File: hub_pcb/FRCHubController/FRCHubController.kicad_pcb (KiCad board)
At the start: 2 copper layers, 60 x 79.5 mm, 20 parts, among them J1 Conn_01x03_Socket, J2 Conn_01x03_Socket, J3 Conn_01x03_Socket, J4 Barrel_Jack_Switch_Pin3Ring, J5 Conn_02x08_Odd_Even, U6 TXB0102DCU

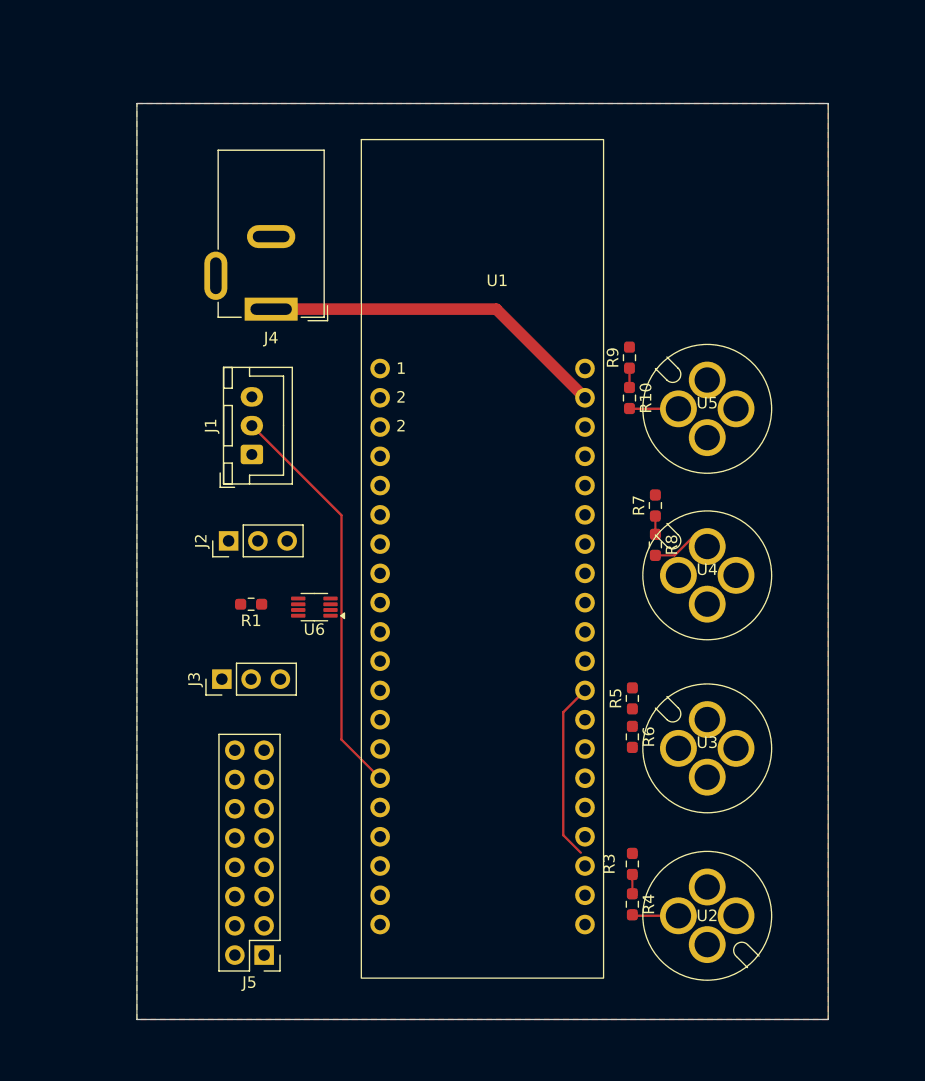
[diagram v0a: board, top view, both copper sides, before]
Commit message: Layout PCB
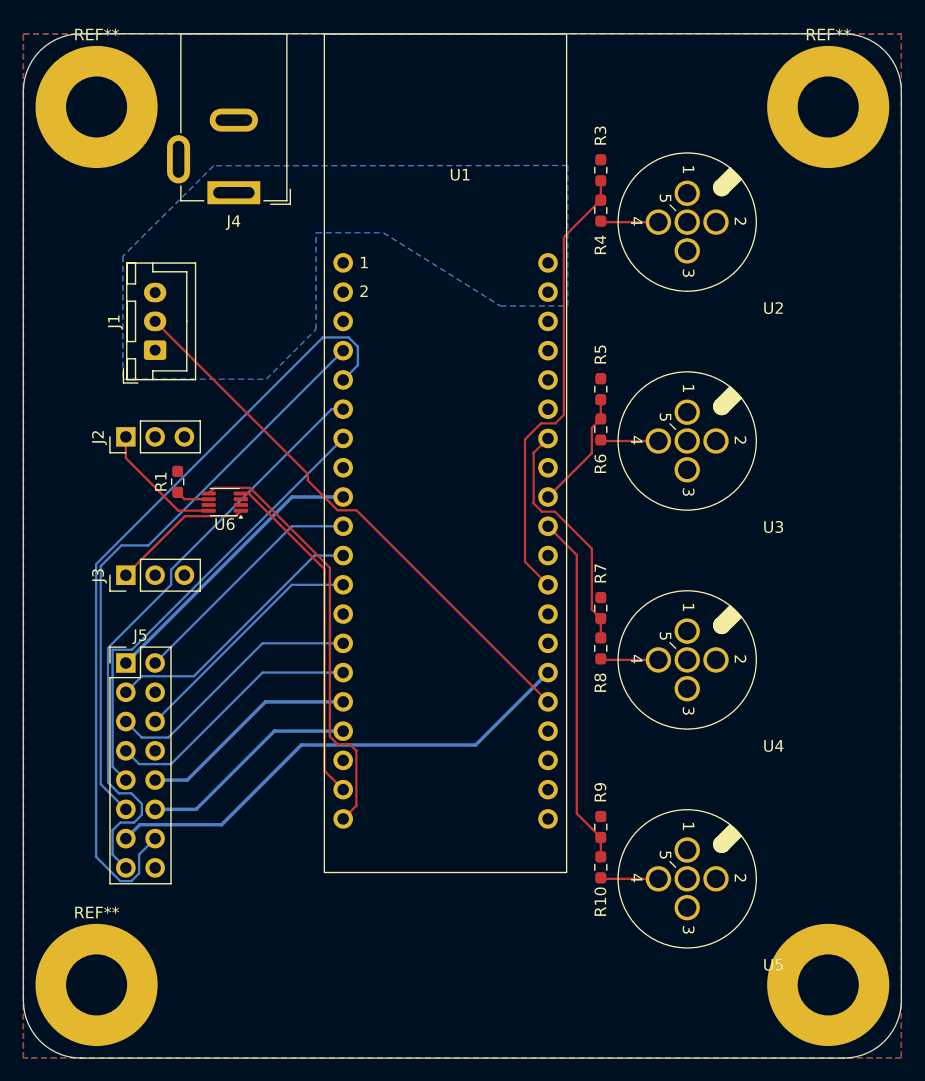
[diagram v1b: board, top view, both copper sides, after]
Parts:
- removed the R10 at (173.2, 76.1)
- removed the R9 at (173.2, 72.6)
- removed the U5 at (180.0, 77.0)
- added ?: , , F.Cu at (190.5, 127.0)
- added R3: 330, Resistor_SMD:R_0603_1608Metric_Pad0.98x0.95mm_HandSolder, F.Cu at (170.8, 56.3)
- added R4: 1K, Resistor_SMD:R_0603_1608Metric_Pad0.98x0.95mm_HandSolder, F.Cu at (170.8, 59.8)
- added REF**: MountingHole_5.3mm_M5_Pad, MountingHole:MountingHole_5.3mm_M5_Pad, F.Cu at (190.5, 50.8)
- added REF**: MountingHole_5.3mm_M5_Pad, MountingHole:MountingHole_5.3mm_M5_Pad, F.Cu at (127.0, 50.8)
- added REF**: MountingHole_5.3mm_M5_Pad, MountingHole:MountingHole_5.3mm_M5_Pad, F.Cu at (127.0, 127.0)
- added U2: ~, Library:M12, F.Cu at (178.3, 60.8)
- moved J5 28.0 mm to (129.5, 99.1), turned to 0 degrees
- moved R5 27.0 mm to (170.8, 75.3)
- moved R6 26.8 mm to (170.8, 78.8)
- moved U3 26.7 mm to (178.3, 79.8), turned to -90 degrees
- moved J2 12.7 mm to (129.5, 79.4)
- moved R1 12.4 mm to (134.0, 83.3), turned to 90 degrees
- moved J1 12.3 mm to (132.1, 71.9)
- moved J3 12.3 mm to (129.5, 91.4)
- moved U6 12.0 mm to (138.1, 85.1)
- moved J4 10.6 mm to (138.9, 58.2)
- moved R8 10.2 mm to (170.8, 97.8)
- moved R7 10.1 mm to (170.8, 94.3)
- moved U1 9.71 mm to (157.3, 64.3)
- moved U4 7.54 mm to (178.3, 98.8), turned to -90 degrees
- moved R10 4.22 mm to (170.8, 116.8)
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- renumbered R4 to R10, R3 to R9, U2 to U5
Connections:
- R10 pad 1: /PHOTOEYE1 -> /PHOTOEYE4
- R9 pad 1: /PHOTOEYE1 -> /PHOTOEYE4
- U1 pad 15: /LED -> /B2
- U1 pad 25: unconnected-(U1-GPIO1-Pad25) -> /LED
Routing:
- net /LAT: track 0.00 -> 68.5 mm
- net /OE: track 0.00 -> 52.9 mm
- net /C: track 0.00 -> 50.8 mm
- net /CLK: track 0.00 -> 42.6 mm
- net /A: track 0.00 -> 39.4 mm
- net /PWM1: track 0.00 -> 37.5 mm
- net +5V: track 30.4 -> 0.00 mm
- net /PWM2: track 0.00 -> 29.8 mm
- net /PHOTOEYE4: track 1.67 -> 30.6 mm
- net /R1: track 0.00 -> 24.8 mm
- net /B1: track 0.00 -> 23.8 mm
- net /R2: track 0.00 -> 22.8 mm
- net /B2: track 0.00 -> 22.6 mm
- net /PHOTOEYE1: track 17.2 -> 39.3 mm
- net /G1: track 0.00 -> 21.2 mm
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- added copper zone on B.Cu, net +5V
- added copper zone on B.Cu, net GND
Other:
- board size 60 x 79.5 mm -> 76.2 x 88.9 mm
